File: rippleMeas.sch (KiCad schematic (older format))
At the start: 25 parts, among them Q1 BC817, Q2 MMST3906, SW1 RST, U10 LMC6482

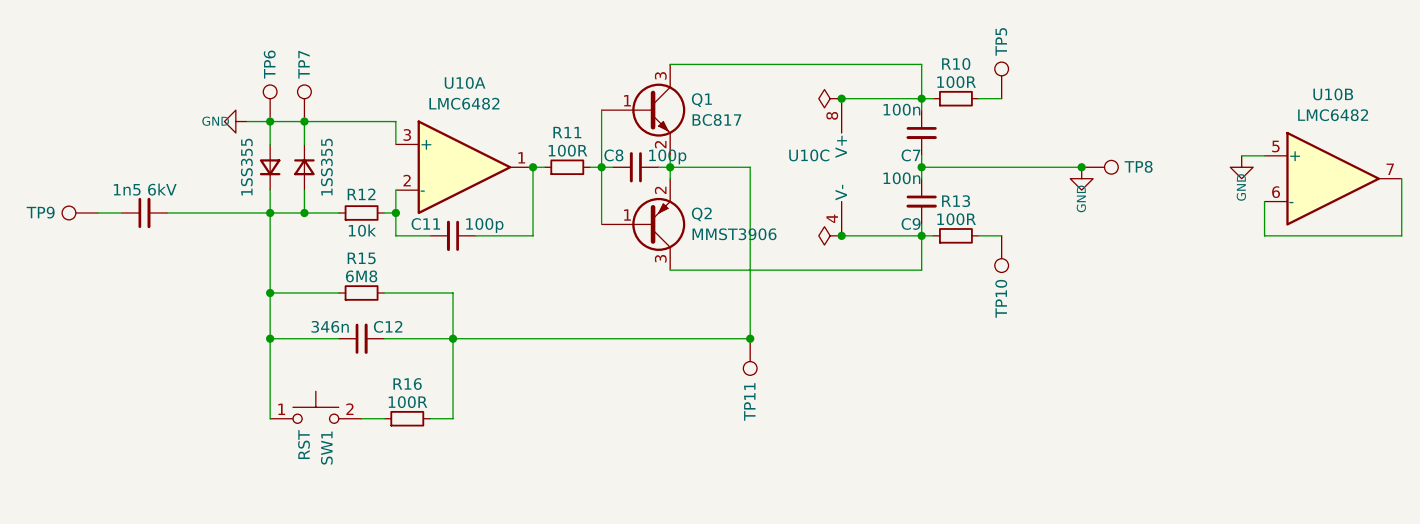
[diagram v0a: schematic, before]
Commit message: - PCB progress
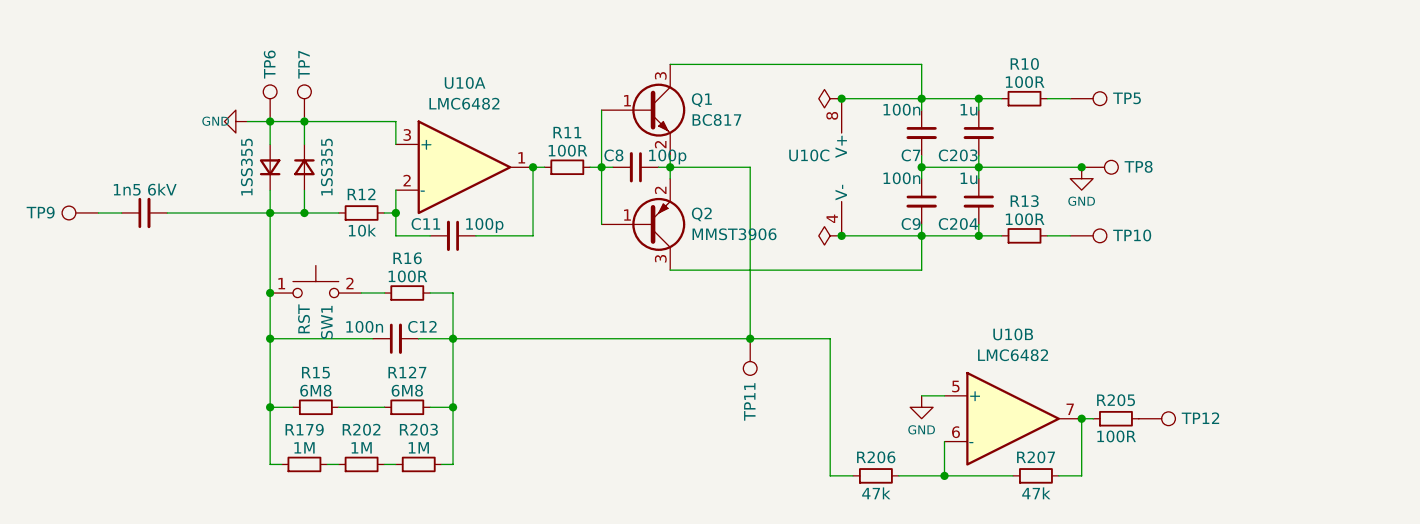
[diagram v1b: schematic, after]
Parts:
- added C203, C204: 1u, Capacitor_SMD:C_0603_1608Metric, symbol Device:C_Small
- added R127: 6M8, Resistor_SMD:R_1206_3216Metric_Pad1.42x1.75mm_HandSolder, symbol Device:R_Small
- added R179, R202, R203: 1M, Resistor_SMD:R_0603_1608Metric_Pad1.05x0.95mm_HandSolder, symbol Device:R_Small
- added R205: 100R, Resistor_SMD:R_0603_1608Metric, symbol Device:R_Small
- added R206, R207: 47k, Resistor_SMD:R_0603_1608Metric, symbol Device:R_Small
- added TP12: TestPoint, TestPoint:TestPoint_THTPad_D1.5mm_Drill0.7mm, symbol Connector:TestPoint
- C11, C7, C8, C9: footprint Capacitor_SMD:C_0603_1608Metric_Pad1.05x0.95mm_HandSolder -> Capacitor_SMD:C_0603_1608Metric
- C12: value 346n -> 100n
- R10, R11, R12, R13, R16: footprint Resistor_SMD:R_0603_1608Metric_Pad1.05x0.95mm_HandSolder -> Resistor_SMD:R_0603_1608Metric
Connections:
- net GND: now also C203.2, C204.1
- net at C10.2, C12.1, D1.1 (K)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: now also R179.1
- net at C12.2, C8.1, Q1.2 (E)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: now also R127.2, R203.2, R206.1; no longer R15.2
- net at U10.6 (-): now also R206.2, R207.1; no longer U10.7
- net at C9.2, Q2.3 (C), R13.1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: now also C204.2
- net at C7.1, Q1.3 (C), R10.1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: now also C203.1
- new net: R127.1, R15.2
- new net: R205.1, R207.2, U10.7
- new net: R179.2, R202.1
- new net: R202.2, R203.1
- new net: R205.2, TP12.1
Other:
- moved on the sheet: C12, R10, R13, R15, R16, SW1, TP10, TP5, U10B
